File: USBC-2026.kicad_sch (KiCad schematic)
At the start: 12 parts, among them IC1 TPS25752ASRSMR, J1 USB_C_Receptacle, U1 TPS55288RPMR

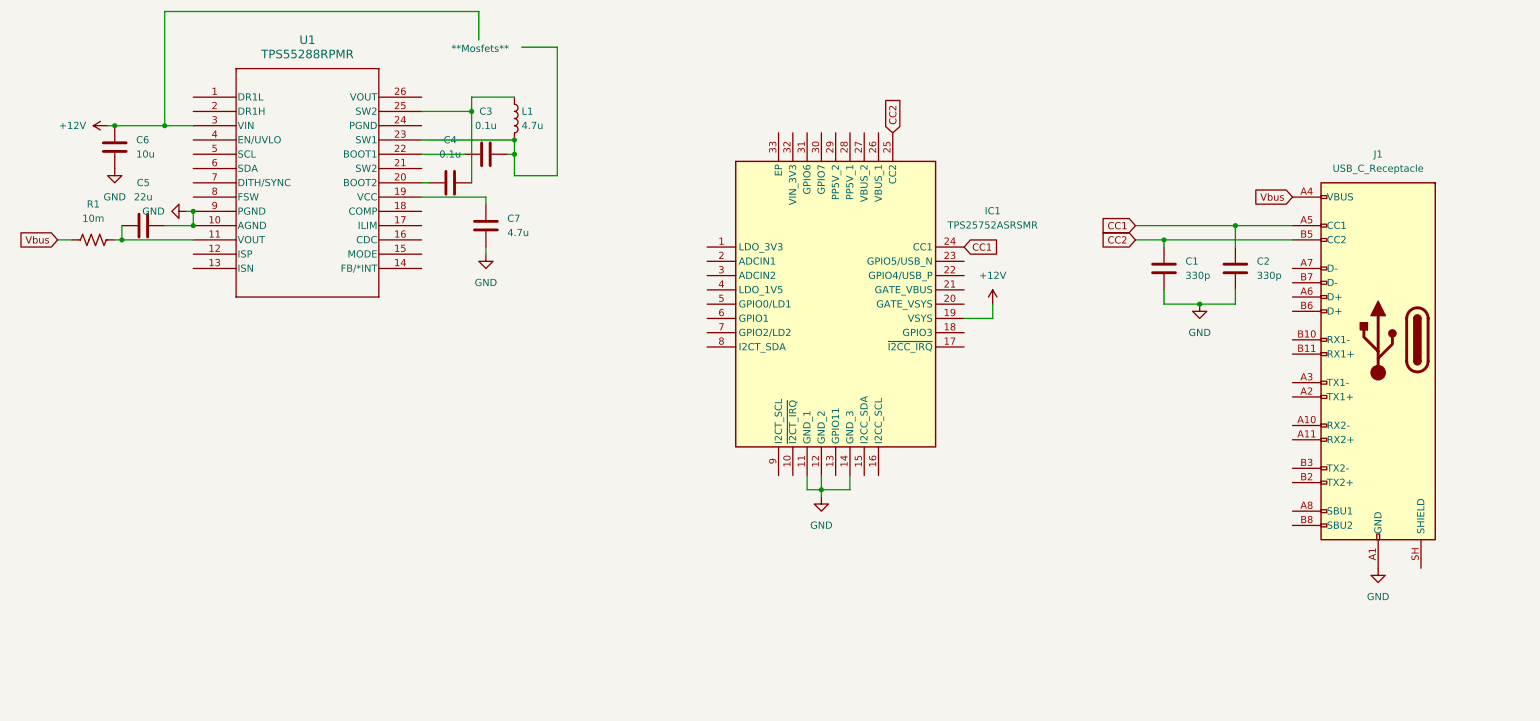
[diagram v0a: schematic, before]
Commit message: Continued work on DC/DC and USB PD Circuits.
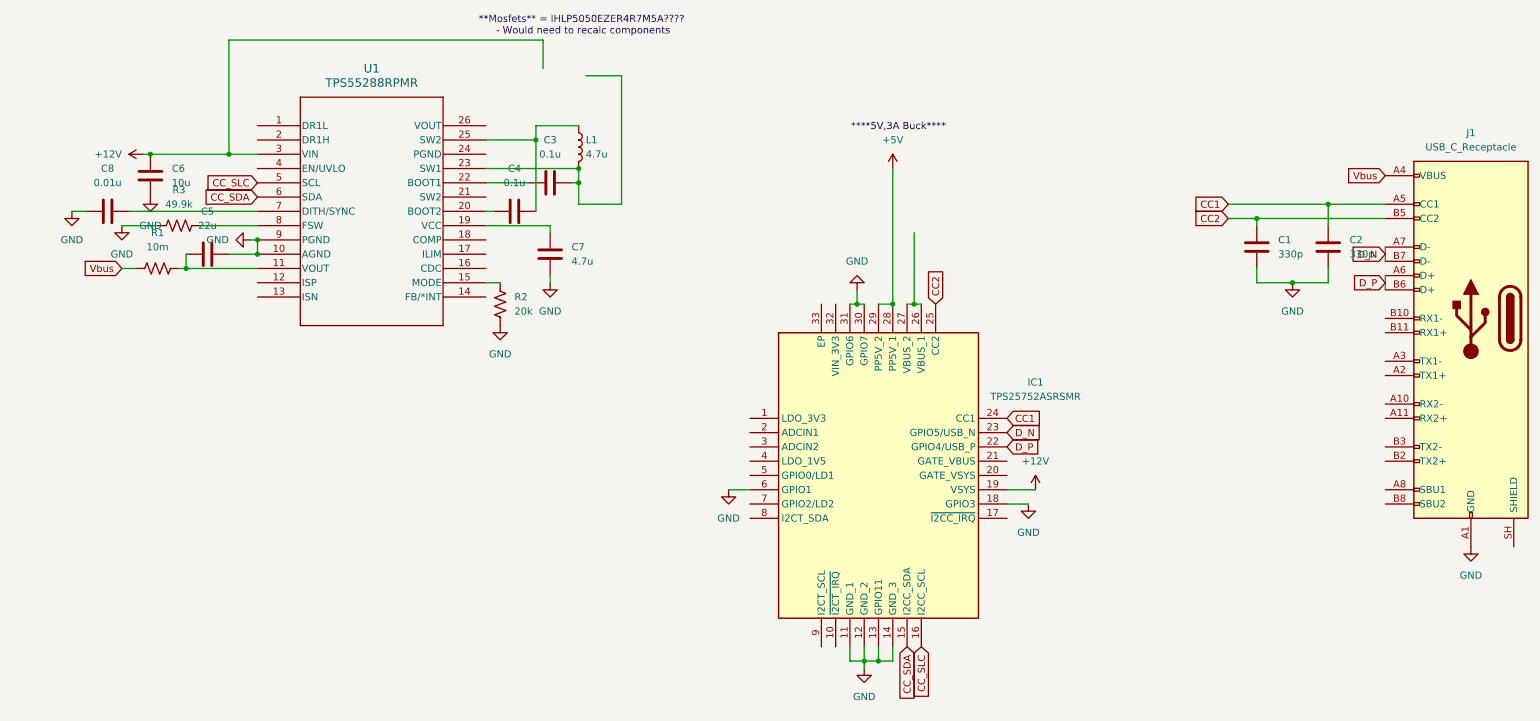
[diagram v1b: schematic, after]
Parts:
- added C8: 0.01u, symbol Device:C
- added R2: 20k, symbol Device:R_US
- added R3: 49.9k, symbol Device:R_US
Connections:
- net GND: now also IC1.13 (GPIO11), IC1.18 (GPIO3), IC1.30 (GPIO7), IC1.31 (GPIO6), IC1.6 (GPIO1), C8.2, R2.1, R3.2
- net D_P: now reaches J1.A6 (D+)
- net D_P: now also IC1.22 (GPIO4/USB_P), J1.B6 (D+)
- net D_N: now reaches J1.A7 (D-)
- net D_N: now also IC1.23 (GPIO5/USB_N), J1.B7 (D-)
- net CC_SDA: now reaches IC1.15 (I2CC_SDA)
- net CC_SDA: now also U1.6 (SDA)
- net CC_SLC: now reaches IC1.16 (I2CC_SCL)
- net CC_SLC: now also U1.5 (SCL)
- net at IC1.26 (VBUS_1): now also IC1.27 (VBUS_2)
- net +5V: now reaches IC1.28 (PP5V_1)
- net +5V: now also IC1.29 (PP5V_2)
- net at U1.15 (MODE): now also R2.2
- net at U1.7 (DITH/SYNC): now also C8.1
- net at U1.8 (FSW): now also R3.1
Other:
- note added: "****5V,3A Buck****"
- note added: "**Mosfets** = IHLP5050EZER4R7M5A???? - Would need to recalc components"
- note removed: "**Mosfets**"
- moved on the sheet: C1, C2, C3, C4, C5, C6, C7, IC1, J1, L1, R1, U1
